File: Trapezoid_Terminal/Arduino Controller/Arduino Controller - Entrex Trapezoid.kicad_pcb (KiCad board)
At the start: 2 copper layers, 114 x 87 mm, 18 parts, among them J1 Conn_01x19, J10 Conn_01x04, J2 Conn_01x04, J3 Conn_01x08, J4 Conn_01x08, J5 Conn_01x06, J6 Conn_01x04, J8 Conn_01x19, J9 Logic 8 CH, U1 74LS04

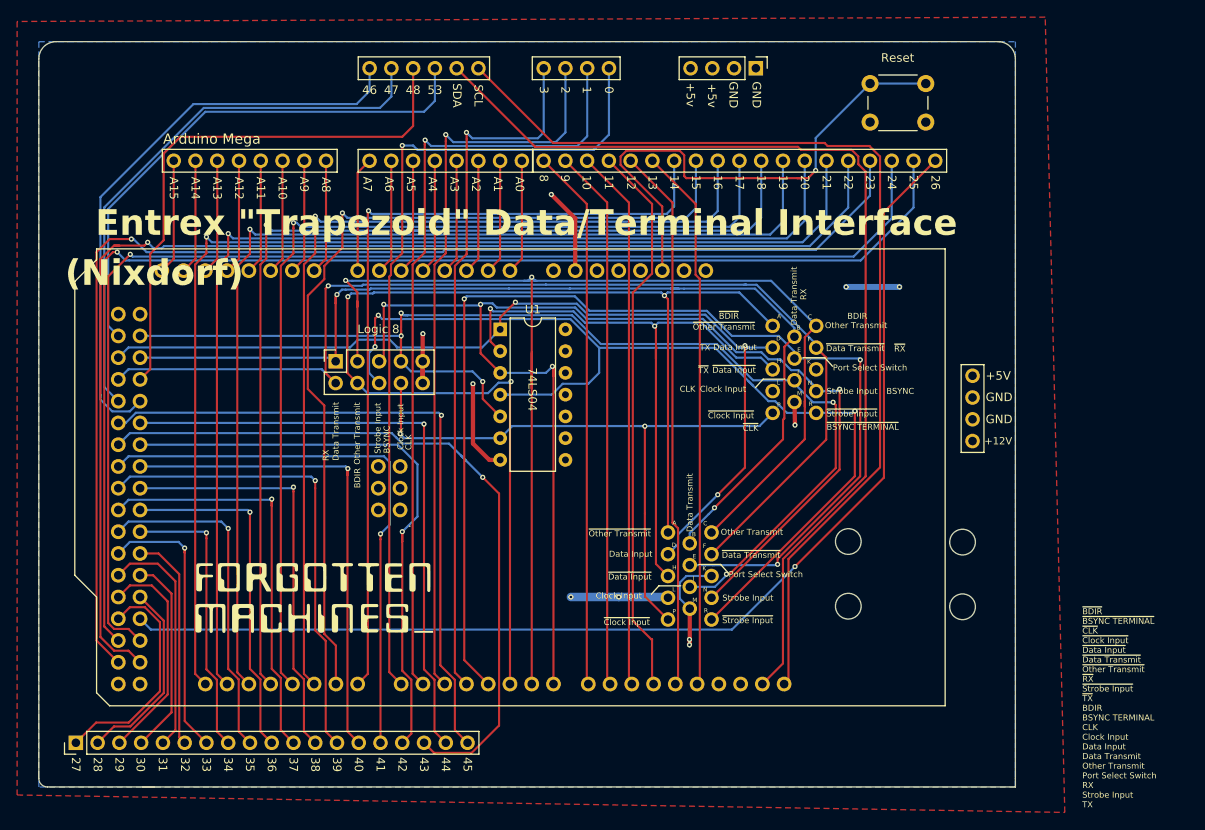
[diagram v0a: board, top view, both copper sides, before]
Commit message: DRC Checks p1
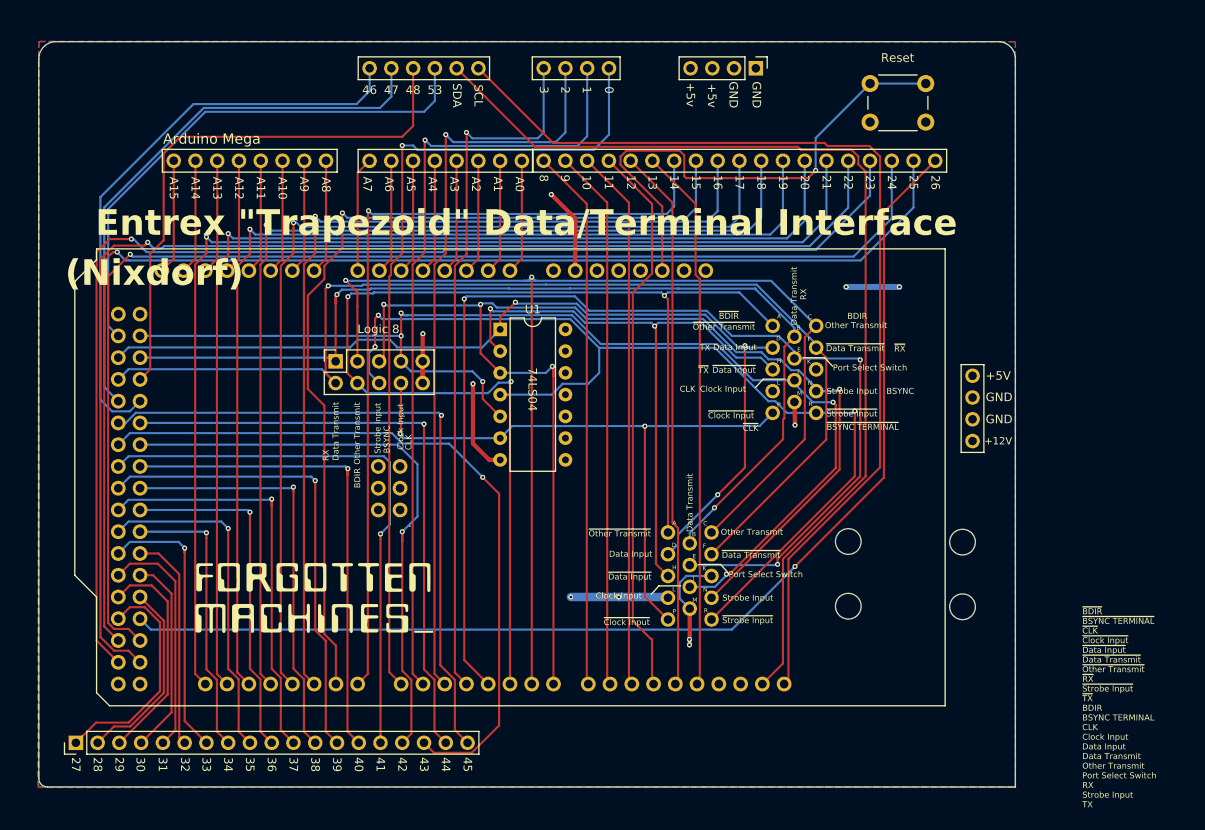
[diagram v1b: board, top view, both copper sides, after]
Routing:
- net Other Transmit: track 151.0 -> 145.6 mm
- net ~{Data Input}: track 72.8 -> 71.5 mm
- net D43: track 86.4 -> 85.6 mm
- net ~{Strobe Input}: track 117.8 -> 117.0 mm
- net Data Transmit: track 118.2 -> 117.5 mm
- net D18: track 120.3 -> 119.7 mm
- net Net-(XA1-RESET): track 61.4 -> 60.9 mm
- net D22: track 146.3 -> 145.8 mm
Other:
- outline, holes or cut-outs redrawn
